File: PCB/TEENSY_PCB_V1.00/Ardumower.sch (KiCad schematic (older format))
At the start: 50 parts, among them J1 ODO_Left, J10 Sonar_R, J11 Cutter, J12 Sonar_L, J13 P_Right, J14 Buzzer, J15 Button, J16 Power_Board, J19 P_Left, J2 I2C2_0, J25 5V IN, J29 3.3V IN, J3 I2C0_0, J30 I2C1_0, J31 Ser3, J4 I2C1_1, J5 Bumper, J6 ODO_Right, J7 Motor_Right1, J8 Motor_Left1, J9 Rain, U1 DOIT-ESP32-DEVKIT-V1, U2 GY-521, U3 Teensy4.1

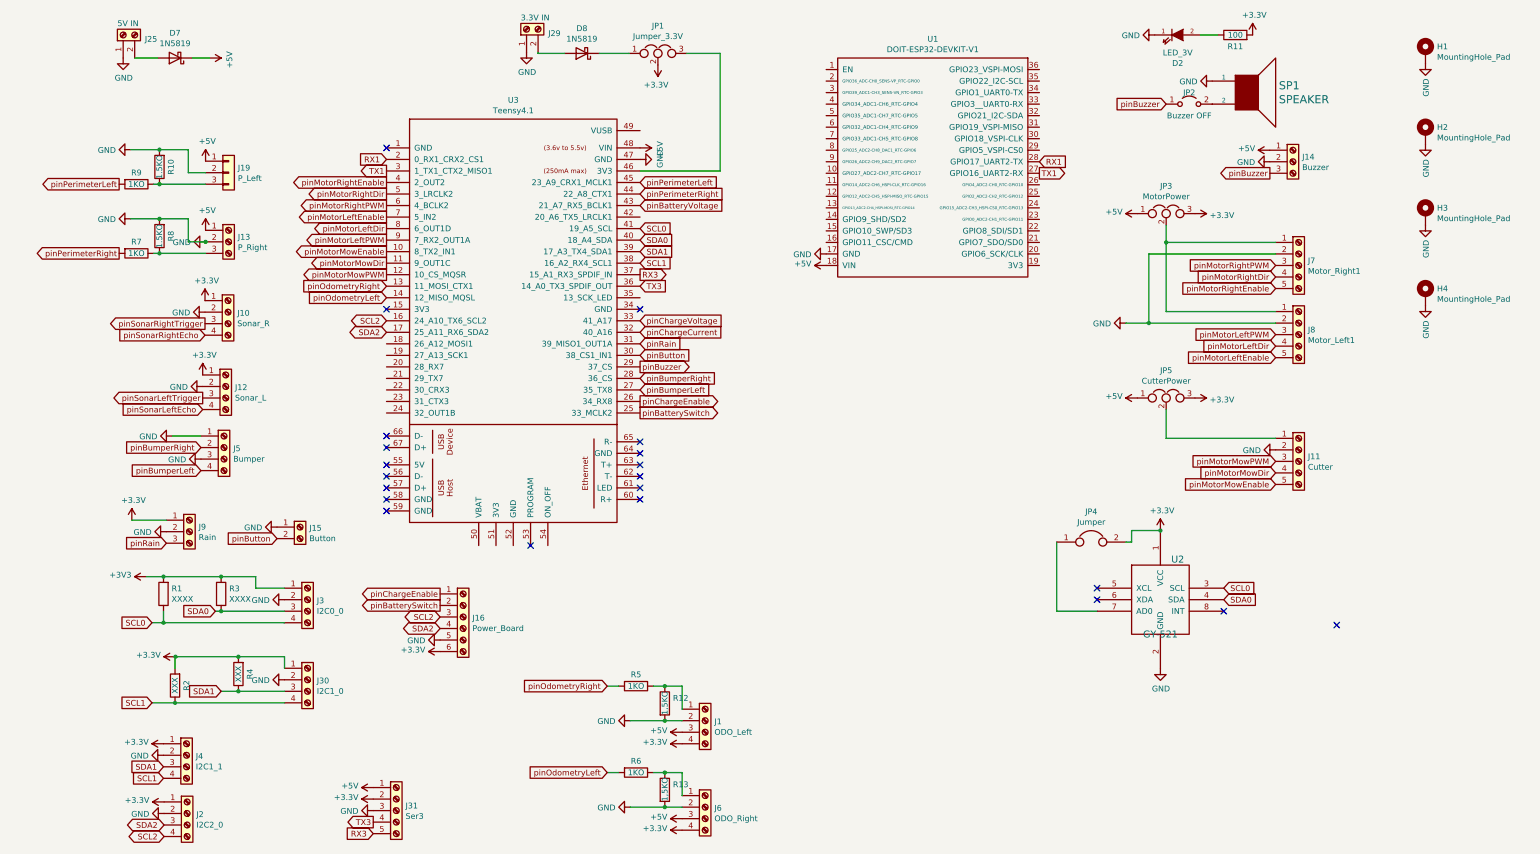
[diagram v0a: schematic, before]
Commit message: test
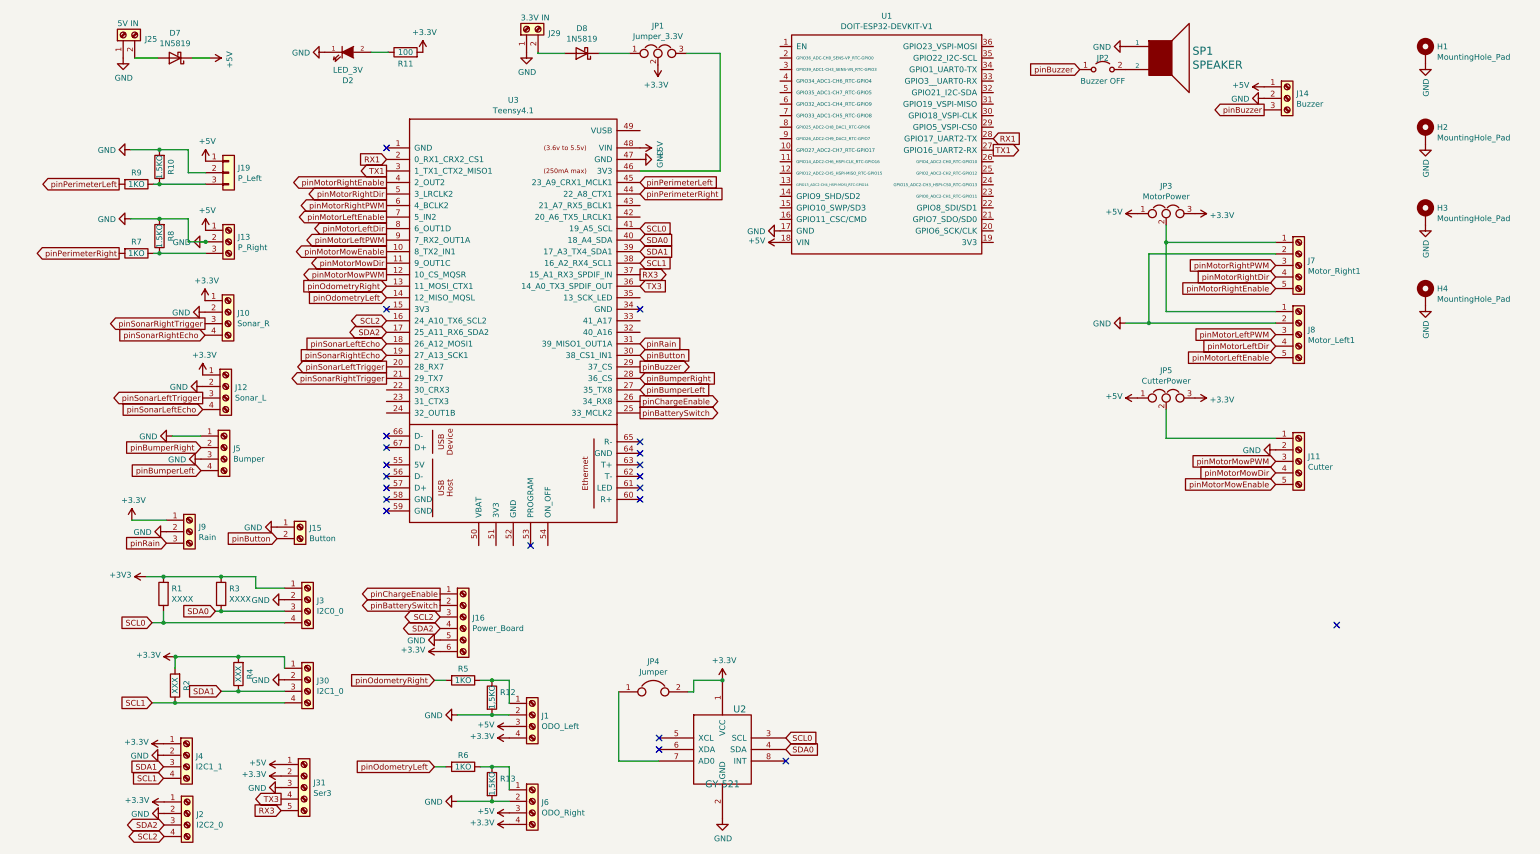
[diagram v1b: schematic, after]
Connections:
- net pinSonarLeftEcho: now also U3.18 (26_A12_MOSI1)
- net pinSonarLeftTrigger: now also U3.20 (28_RX7)
- net pinSonarRightEcho: now also U3.19 (27_A13_SCK1)
- net pinSonarRightTrigger: now also U3.21 (29_TX7)
- net pinBatteryVoltage: no longer names the net of U3.43 (21_A7_RX5_BCLK1)
- net pinChargeCurrent: no longer names the net of U3.32 (40_A16)
- net pinChargeVoltage: no longer names the net of U3.33 (41_A17)
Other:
- moved on the sheet: D2, J1, J14, J31, J6, JP2, JP4, R11, R12, R13, R5, R6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
